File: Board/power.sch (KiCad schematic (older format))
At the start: 20 parts, among them U1 TPS54531

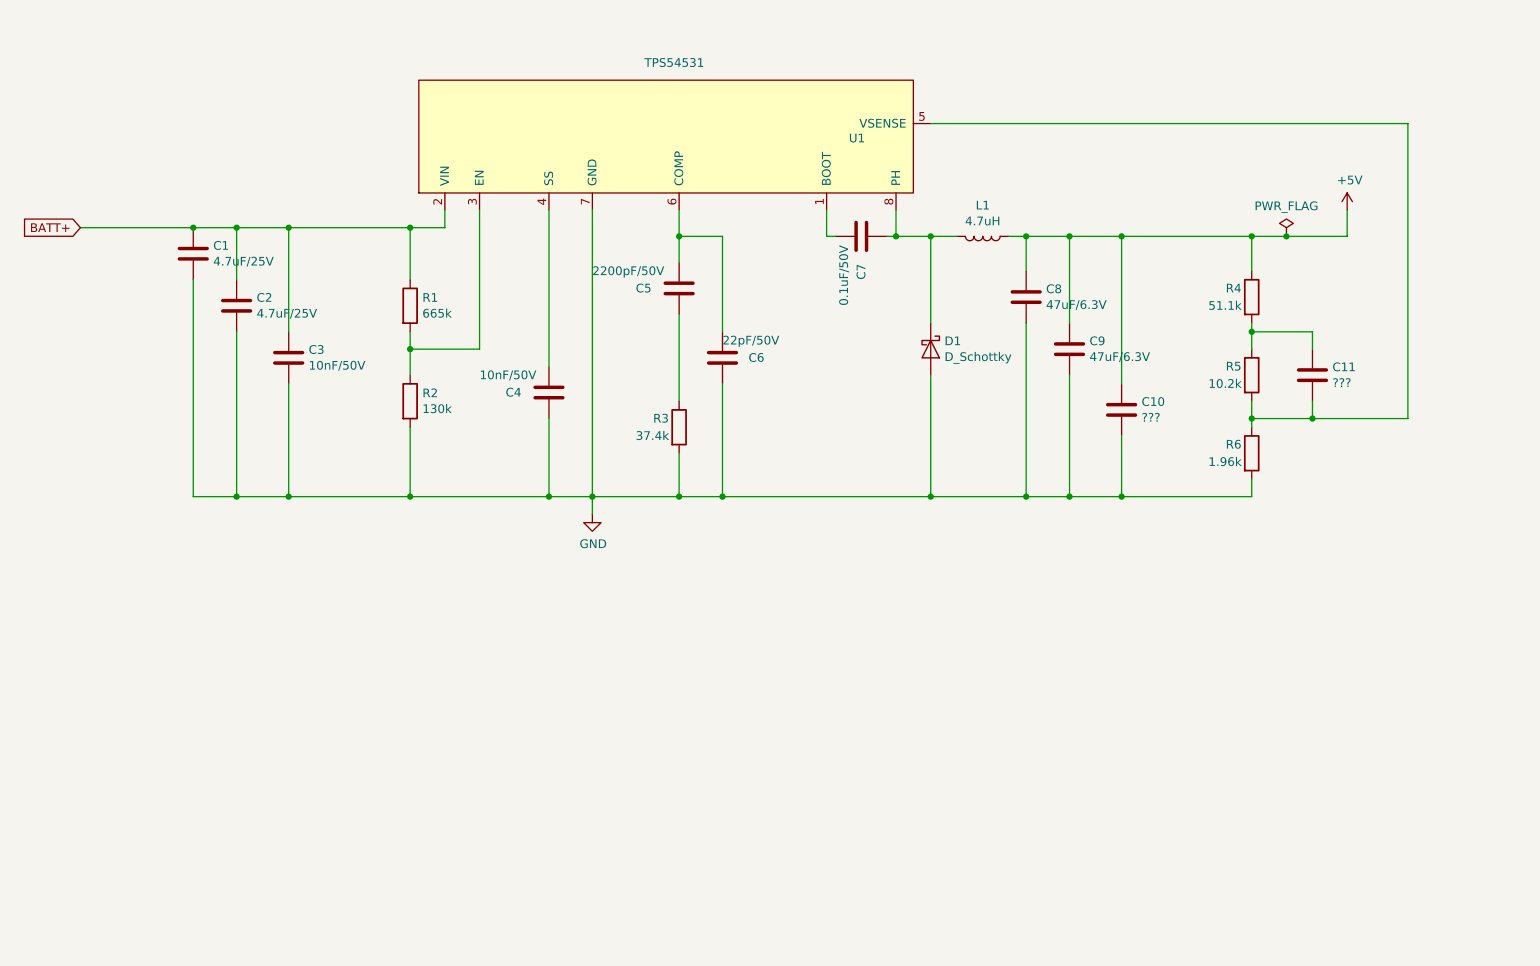
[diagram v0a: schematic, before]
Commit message: Routing done.
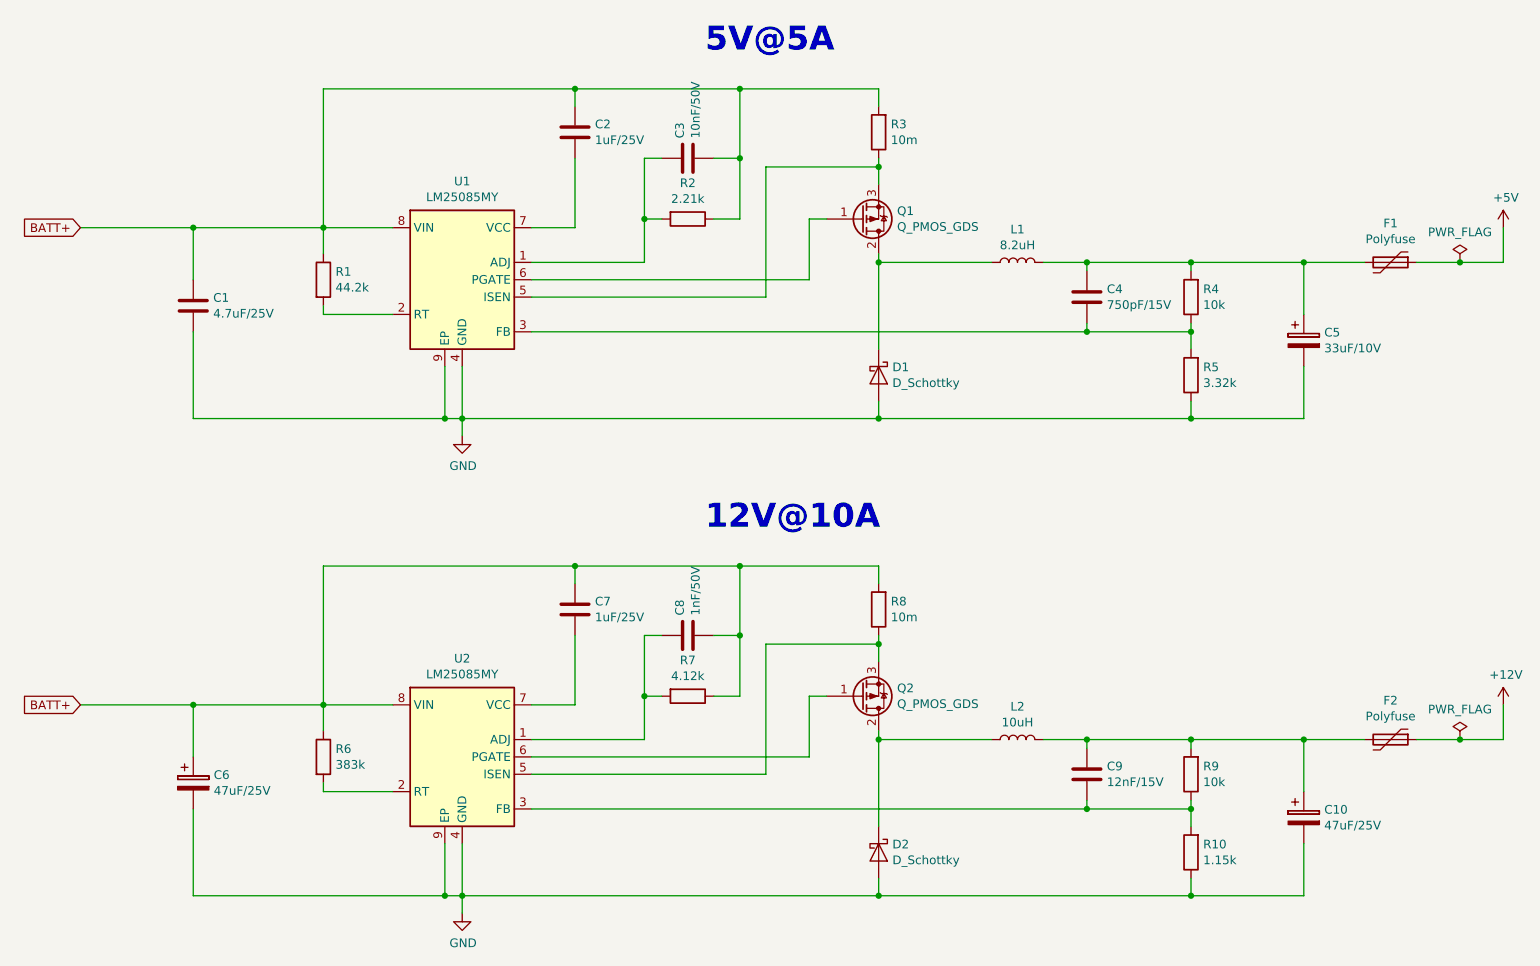
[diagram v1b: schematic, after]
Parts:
- removed C10, C11: ???, symbol Device:C
- removed C5: 2200pF/50V, symbol Device:C
- removed C6: 22pF/50V, symbol Device:C
- removed U1: TPS54531, symbol power_custom:TPS54531
- added C10, C6: 47uF/25V, symbol Device:CP
- added C5: 33uF/10V, symbol Device:CP
- added D2: D_Schottky, symbol Device:D_Schottky
- added F1, F2: Polyfuse, symbol Device:Polyfuse
- added L2: 10uH, symbol Device:L
- added Q1, Q2: Q_PMOS_GDS, Package_TO_SOT_SMD:TO-263-2, symbol Device:Q_PMOS_GDS
- added R10: 1.15k, symbol Device:R
- added R7: 4.12k, symbol Device:R
- added R8: 10m, Resistor_SMD:R_1206_3216Metric_Pad1.42x1.75mm_HandSolder, symbol Device:R
- added R9: 10k, symbol Device:R
- added U1, U2: LM25085MY, Package_SO:MSOP-8-1EP_3x3mm_P0.65mm_EP1.68x1.88mm, symbol Regulator_Switching:LM25085MY
- C2: value 4.7uF/25V -> 1uF/25V
- C4: value 10nF/50V -> 750pF/15V
- C7: value 0.1uF/50V -> 1uF/25V
- C8: value 47uF/6.3V -> 1nF/50V
- C9: value 47uF/6.3V -> 12nF/15V
- D1: footprint Diode_SMD:D_SMC_Handsoldering -> (none); Farnell 1843671 -> 2773825; Ref B540C-13-F -> MBRD10200CT
- L1: value 4.7uH -> 8.2uH; Farnell 2077823 -> 2289089; Ref 74437368047 -> XAL6060-822MEC
- R1: value 665k -> 44.2k
- R2: value 130k -> 2.21k
- R3: value 37.4k -> 10m; footprint (none) -> Resistor_SMD:R_1206_3216Metric_Pad1.42x1.75mm_HandSolder; Farnell (none) -> 1099907; Ref (none) -> LRF1206-R01FW
- R4: value 51.1k -> 10k
- R5: value 10.2k -> 3.32k
- R6: value 1.96k -> 383k
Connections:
- net +5V: now also F1.1; no longer C8.1, C9.1, L1.1, R4.1
- net BATT+: now also C3.2, C7.1, C8.2, R2.1, R3.2, R6.1, C6.1, R7.1, R8.2, U1.8 (VIN), U2.8 (VIN); no longer C3.1
- net GND: now also R5.1, C10.2, C5.2, C6.2, D2.2 (A), R10.1, U1.4 (GND), U1.9 (EP), U2.4 (GND), U2.9 (EP); no longer C2.2, C3.2, C4.1, C8.2, C9.2, R2.2, R3.2, R6.2
- net at C7.2: now also U2.7 (VCC)
- net at R1.2: now also U1.2 (RT); no longer R2.1
- net at C4.2: now also R4.1, R5.2, U1.3 (FB)
- net at R3.1: now also Q1.3 (S), U1.5 (ISEN)
- net at R4.2: now also C4.1, L1.2, C5.1, F1.2; no longer R5.1
- new net: C3.1, R2.2, U1.1 (ADJ)
- new net: Q1.1 (G), U1.6 (PGATE)
- new net: C2.2, U1.7 (VCC)
- new net: D1.1 (K), L1.1, Q1.2 (D)
- new net: C8.1, R7.2, U2.1 (ADJ)
- new net: R6.2, U2.2 (RT)
- new net: C9.2, R10.2, R9.1, U2.3 (FB)
- new net: Q2.3 (S), R8.1, U2.5 (ISEN)
- new net: Q2.1 (G), U2.6 (PGATE)
- new net: D2.1 (K), L2.1, Q2.2 (D)
- new net: C10.1, C9.1, F2.2, L2.2, R9.2
- new net +12V: F2.1
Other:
- note added: "12V@10A"
- note added: "5V@5A"
- moved on the sheet: C1
